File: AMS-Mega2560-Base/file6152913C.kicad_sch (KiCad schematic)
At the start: 43 parts, among them IC14 LTV-814, IC15 LTV-814, IC16 LTV-814, IC17 DS3231SN#, IC18 MAX232CPE+, Q10 2N7000, Q11 PSMP033-60YEX, Q12 PSMP033-60YEX, Q13 PSMP033-60YEX, Q5 2N7000, Q6 2N7000, Q7 2N7000, Q8 2N7000, Q9 2N7000, U3 S8411-45R

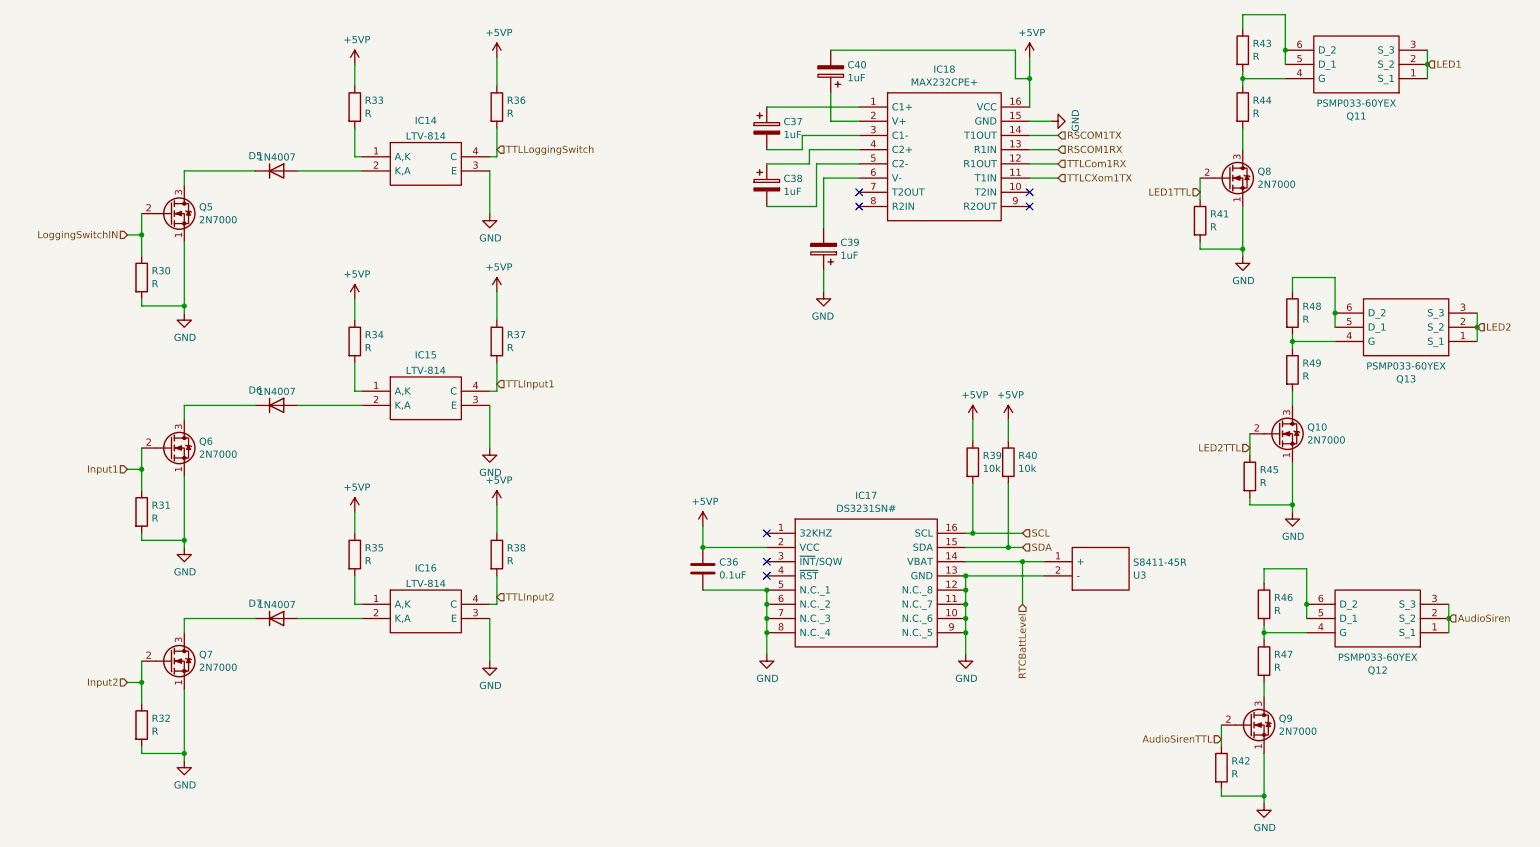
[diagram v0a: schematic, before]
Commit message: BaseBoard fixes and updates. doing schematic work.
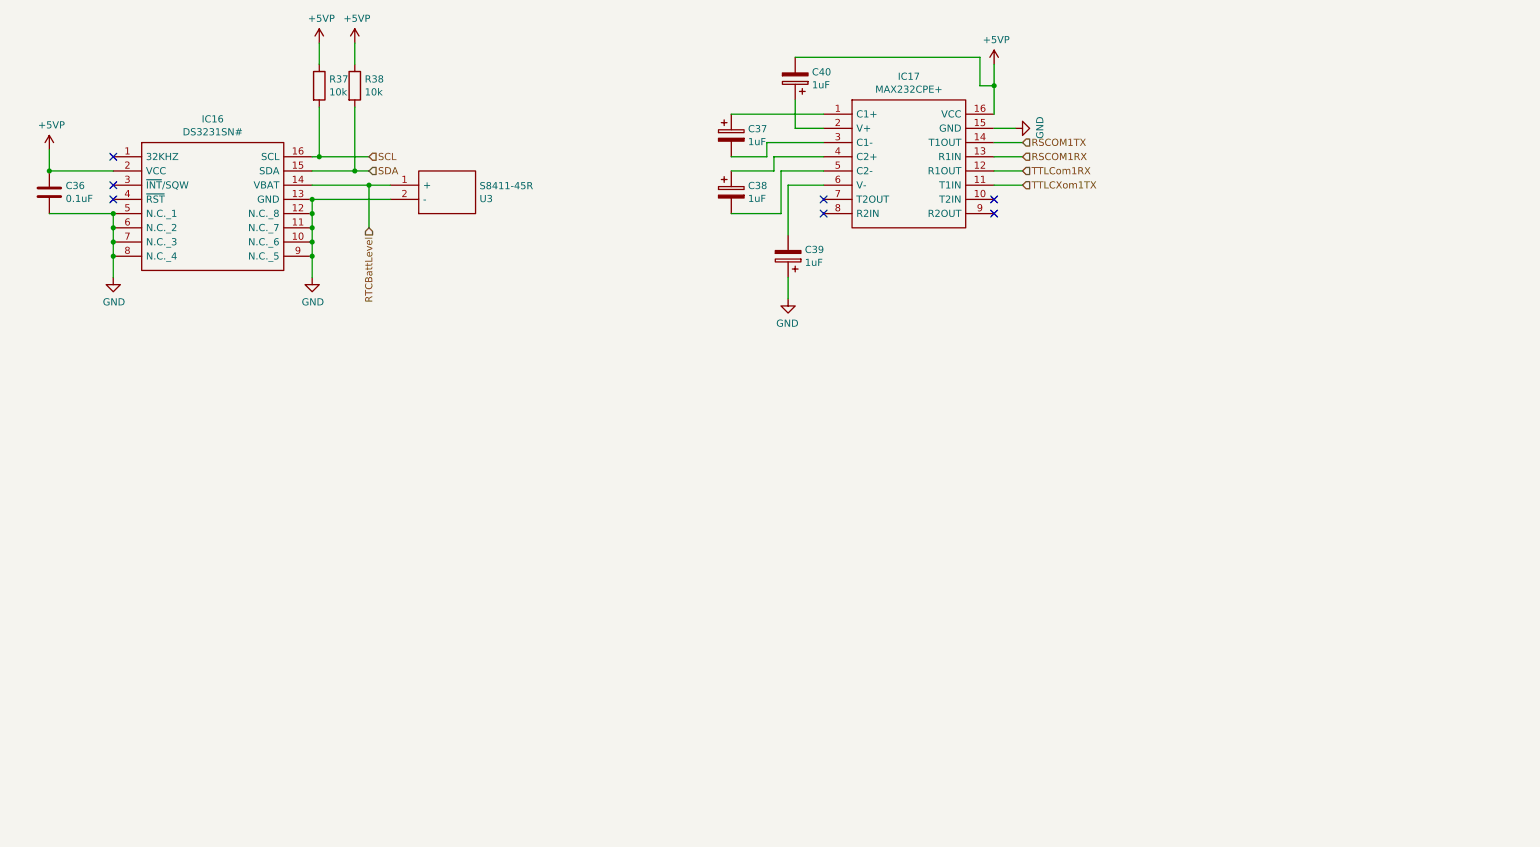
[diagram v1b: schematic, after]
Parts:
- removed D5, D6, D7: 1N4007, Diode_THT:D_DO-41_SOD81_P10.16mm_Horizontal, symbol Diode:1N4007
- removed IC14, IC15, IC16: LTV-814, SamacSys_Parts:DIP762W60P254L460H450Q4N, symbol Samac_Sys:LTV-814
- removed Q10, Q5, Q6, Q7, Q8, Q9: 2N7000, Package_TO_SOT_THT:TO-92_Inline, symbol Transistor_FET:2N7000
- removed Q11, Q12, Q13: PSMP033-60YEX, SamacSys_Parts:PSMP03360YEX, symbol SamacSys_Parts:PSMP033-60YEX
- removed R30, R31, R32, R33, R34, R35, R36, R37, R38, R41, R42, R43, R44, R45, R46, R47, R48, R49: R, Resistor_THT:R_Axial_DIN0207_L6.3mm_D2.5mm_P2.54mm_Vertical, symbol Device:R
- renumbered IC17 to IC16, IC18 to IC17, R39 to R37, R40 to R38
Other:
- moved on the sheet: C36, C37, C38, C39, C40, IC16, IC17, R37, R38, U3
